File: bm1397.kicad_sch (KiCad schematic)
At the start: 58 parts, among them IC1 BM1397_mode1, J3 Conn_01x05, U1 25MHz, U2 TXB0104RGYR, U3 SN74AXC1T45DBVR, U5 MCP1824T-1802E, U6 MCP1824T-0802E

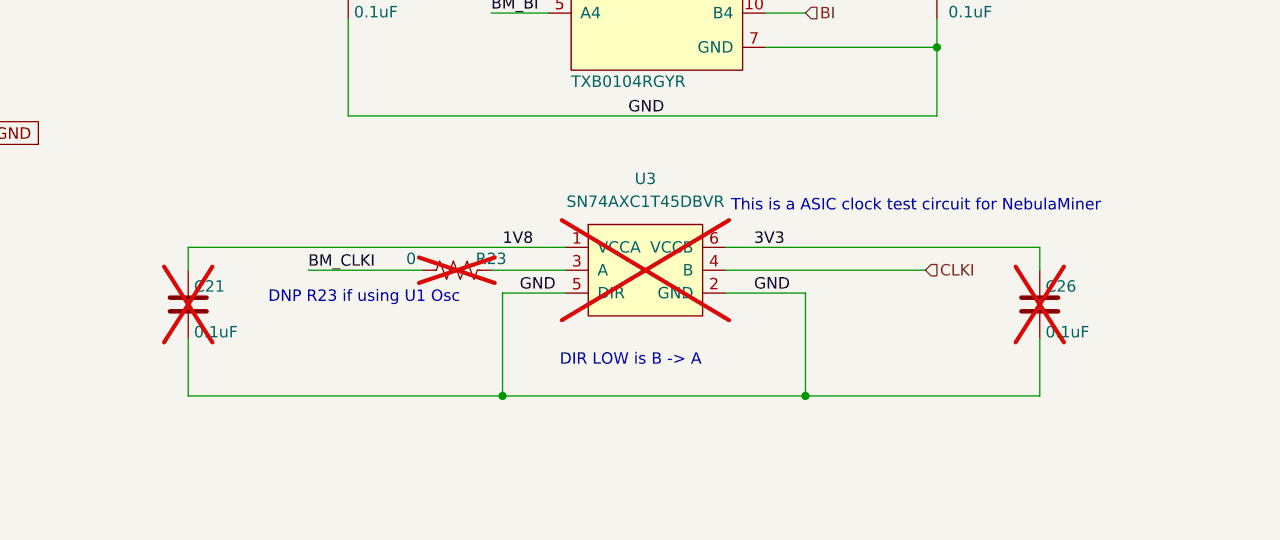
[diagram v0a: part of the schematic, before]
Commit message: Add files via upload
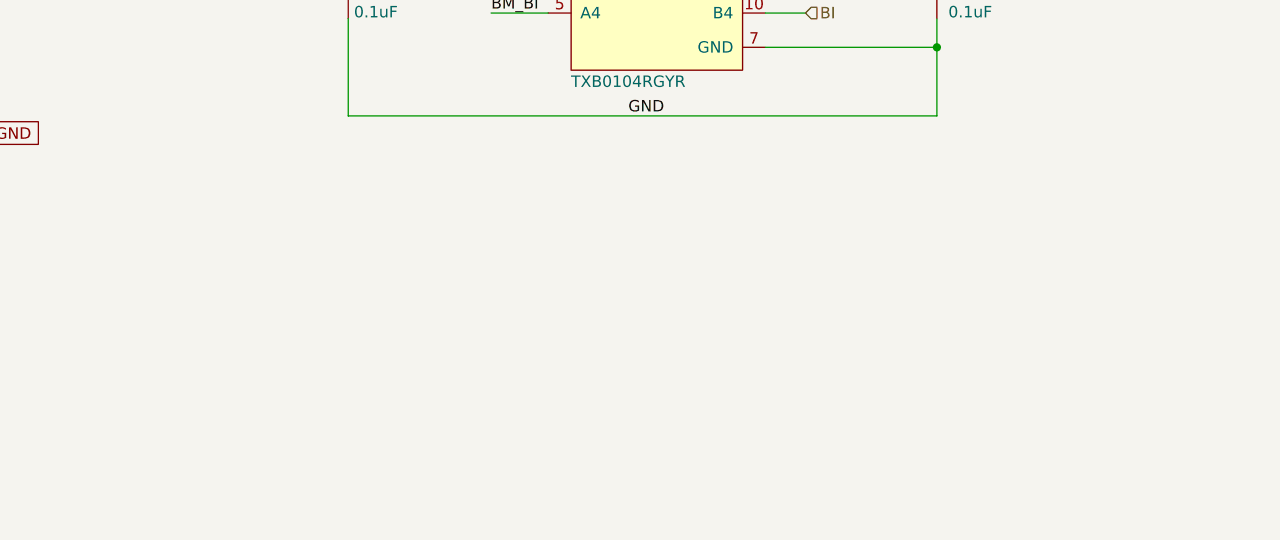
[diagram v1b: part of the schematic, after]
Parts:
- removed C21, C26: 0.1uF, Capacitor_SMD:C_0402_1005Metric, symbol Device:C
- removed R23: 0, Resistor_SMD:R_0402_1005Metric, symbol Device:R_US
- removed U3: SN74AXC1T45DBVR, bitaxe:SN74AXC1T45, symbol bitaxe:SN74AXC1T45DBVR
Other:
- note removed: "DIR LOW is B -> A"
- note removed: "DNP R23 if using U1 Osc"
- note removed: "This is a ASIC clock test circuit for NebulaMiner"
